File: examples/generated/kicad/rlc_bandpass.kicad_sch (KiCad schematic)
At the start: 5 parts

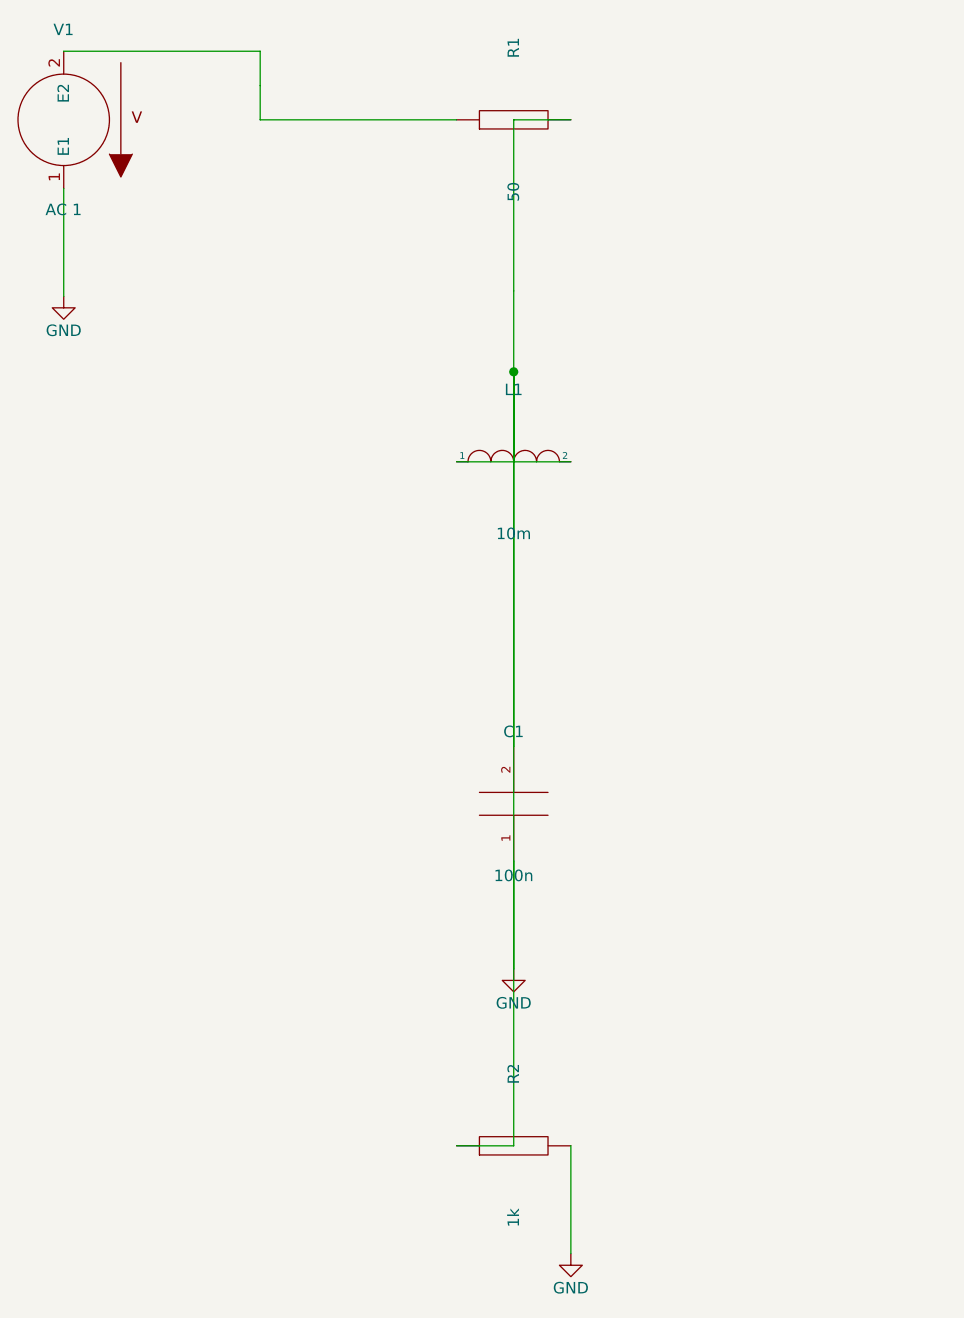
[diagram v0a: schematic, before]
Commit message: Attempt to correct strange wiring.
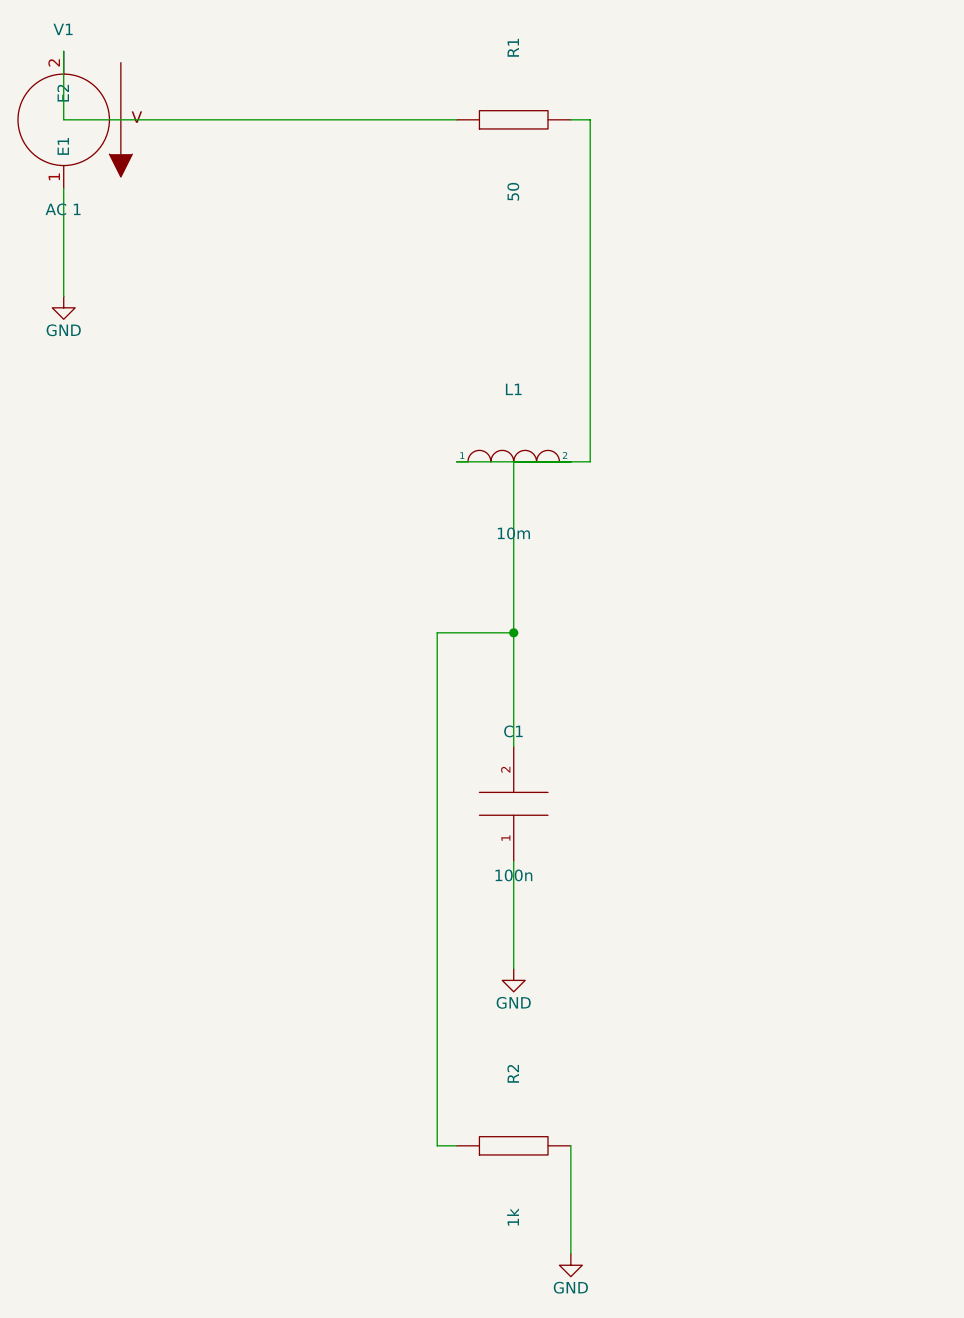
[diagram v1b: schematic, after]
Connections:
- net GND: no longer C1.2, L1.1, L1.2, R1.2, R2.1
- new net: C1.2, L1.1, L1.2, R1.2, R2.1
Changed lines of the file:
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@@
     (stroke (width 0) (type solid) (color 0 0 0 0))
   )
-  (wire (pts (xy 106.35 70.00) (xy 100.00 70.00))
+  (wire (pts (xy 106.35 70.00) (xy 108.50 70.00))
     (stroke (width 0) (type solid) (color 0 0 0 0))
   )
-  (wire (pts (xy 100.00 70.00) (xy 100.00 89.00))
+  (wire (pts (xy 108.50 70.00) (xy 108.50 108.00))
     (stroke (width 0) (type solid) (color 0 0 0 0))
   )
-  (wire (pts (xy 93.65 108.00) (xy 100.00 108.00))
-    (stroke (width 0) (type solid) (color 0 0 0 0))
-  )
-  (wire (pts (xy 100.00 108.00) (xy 100.00 89.00))
+  (wire (pts (xy 108.50 108.00) (xy 93.65 108.00))
     (stroke (width 0) (type solid) (color 0 0 0 0))
   )
@@
     (stroke (width 0) (type solid) (color 0 0 0 0))
   )
-  (wire (pts (xy 100.00 108.00) (xy 100.00 98.00))
+  (wire (pts (xy 100.00 108.00) (xy 100.00 127.00))
     (stroke (width 0) (type solid) (color 0 0 0 0))
   )
-  (wire (pts (xy 100.00 139.65) (xy 100.00 98.00))
+  (wire (pts (xy 100.00 139.65) (xy 100.00 127.00))
     (stroke (width 0) (type solid) (color 0 0 0 0))
   )
-  (wire (pts (xy 93.65 184.00) (xy 100.00 184.00))
+  (wire (pts (xy 93.65 184.00) (xy 91.50 184.00))
     (stroke (width 0) (type solid) (color 0 0 0 0))
   )
-  (wire (pts (xy 100.00 184.00) (xy 100.00 98.00))
+  (wire (pts (xy 91.50 184.00) (xy 91.50 127.00))
     (stroke (width 0) (type solid) (color 0 0 0 0))
   )
-  (wire (pts (xy 50.00 62.38) (xy 71.83 62.38))
+  (wire (pts (xy 91.50 127.00) (xy 100.00 127.00))
     (stroke (width 0) (type solid) (color 0 0 0 0))
   )
-  (wire (pts (xy 71.83 62.38) (xy 71.83 66.19))
+  (wire (pts (xy 50.00 62.38) (xy 50.00 70.00))
     (stroke (width 0) (type solid) (color 0 0 0 0))
   )
-  (wire (pts (xy 93.65 70.00) (xy 71.83 70.00))
+  (wire (pts (xy 50.00 70.00) (xy 93.65 70.00))
     (stroke (width 0) (type solid) (color 0 0 0 0))
   )
-  (wire (pts (xy 71.83 70.00) (xy 71.83 66.19))
-    (stroke (width 0) (type solid) (color 0 0 0 0))
-  )
-  (junction (at 100.00 98.00) (diameter 1.016) (color 0 0 0 0))
+  (junction (at 100.00 127.00) (diameter 1.016) (color 0 0 0 0))
   (sheet_instances
     (path "/" (page "1"))

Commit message: Attempt shape and wiring fixes again.
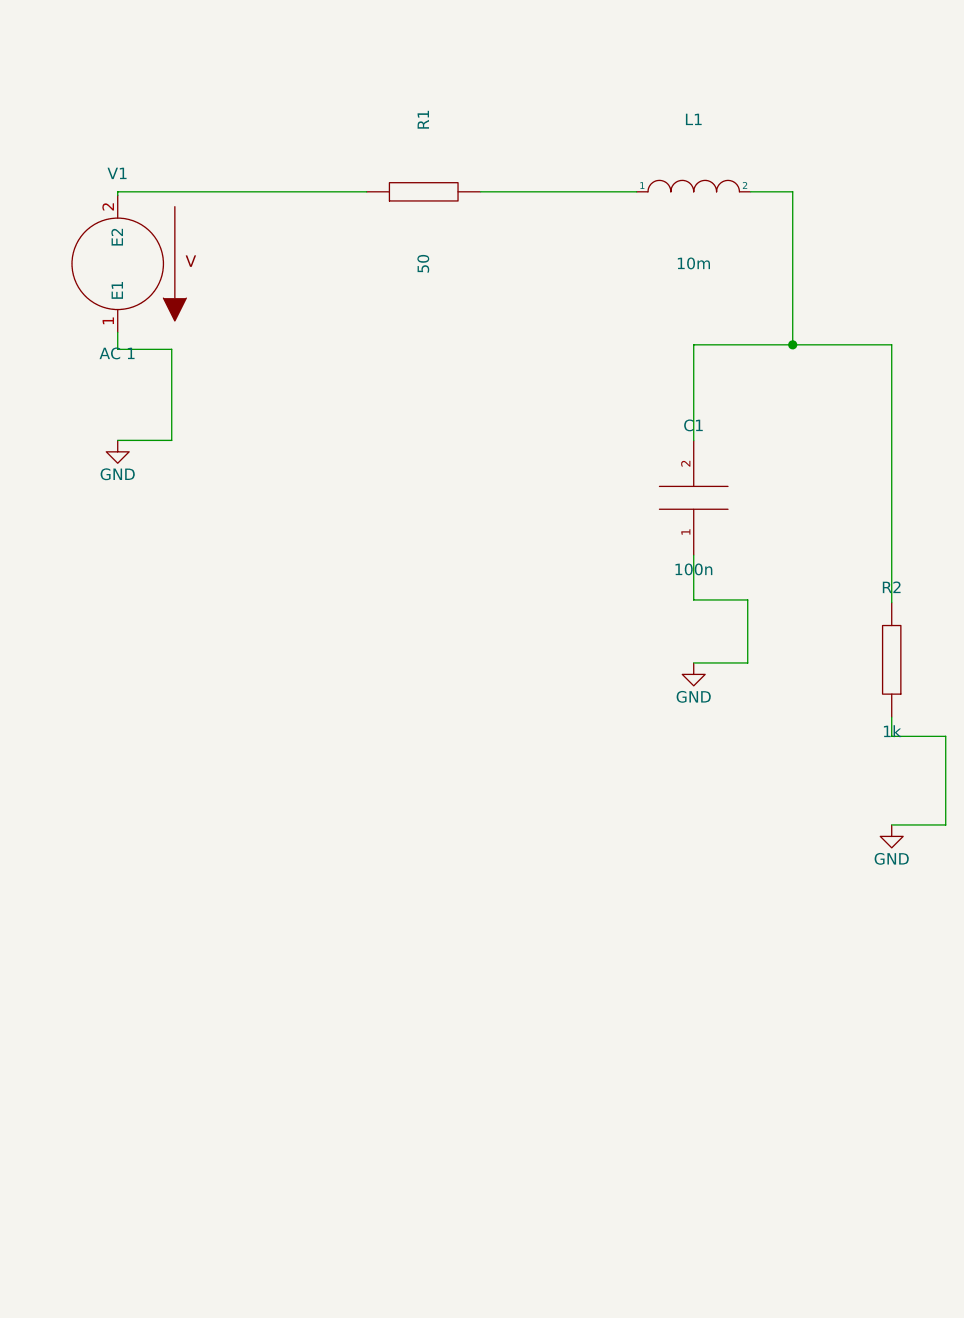
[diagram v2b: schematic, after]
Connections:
- net GND: now also R2.1; no longer R2.2
- new net: L1.1, R1.2
- new net: C1.2, L1.2, R2.2
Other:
- moved on the sheet: C1, L1, R1, R2, V1
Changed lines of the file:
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@@
     (comment 1 "Generated by mixedsig2cad")
   )
-  (symbol (lib_id "VSOURCE") (at 50.00 70.00 180) (unit 1)
+  (symbol (lib_id "VSOURCE") (at 56.00 86.00 180) (unit 1)
     (in_bom yes) (on_board yes)
-    (property "Reference" "V1" (at 50.0 60.0 0)
+    (property "Reference" "V1" (at 56.0 76.0 0)
       (effects (font (size 1.27 1.27)))
     )
-    (property "Value" "AC 1" (at 50.0 80.0 0)
+    (property "Value" "AC 1" (at 56.0 96.0 0)
       (effects (font (size 1.27 1.27)))
     )
@@
     )
   )
-  (symbol (lib_id "R") (at 100.00 70.00 90) (unit 1)
+  (symbol (lib_id "R") (at 90.00 78.00 90) (unit 1)
     (in_bom yes) (on_board yes)
-    (property "Reference" "R1" (at 100.0 62.0 0)
+    (property "Reference" "R1" (at 90.0 70.0 0)
       (effects (font (size 1.27 1.27)))
     )
-    (property "Value" "50" (at 100.0 78.0 0)
+    (property "Value" "50" (at 90.0 86.0 0)
       (effects (font (size 1.27 1.27)))
     )
@@
     )
   )
-  (symbol (lib_id "INDUCTOR") (at 100.00 108.00 0) (unit 1)
+  (symbol (lib_id "INDUCTOR") (at 120.00 78.00 0) (unit 1)
     (in_bom yes) (on_board yes)
-    (property "Reference" "L1" (at 100.0 100.0 0)
+    (property "Reference" "L1" (at 120.0 70.0 0)
       (effects (font (size 1.27 1.27)))
     )
-    (property "Value" "10m" (at 100.0 116.0 0)
+    (property "Value" "10m" (at 120.0 86.0 0)
       (effects (font (size 1.27 1.27)))
     )
@@
     )
   )
-  (symbol (lib_id "CAP") (at 100.00 146.00 180) (unit 1)
+  (symbol (lib_id "CAP") (at 120.00 112.00 180) (unit 1)
     (in_bom yes) (on_board yes)
-    (property "Reference" "C1" (at 100.0 138.0 0)
+    (property "Reference" "C1" (at 120.0 104.0 0)
       (effects (font (size 1.27 1.27)))
     )
-    (property "Value" "100n" (at 100.0 154.0 0)
+    (property "Value" "100n" (at 120.0 120.0 0)
       (effects (font (size 1.27 1.27)))
     )
@@
     )
   )
-  (symbol (lib_id "R") (at 100.00 184.00 90) (unit 1)
+  (symbol (lib_id "R") (at 142.00 130.00 180) (unit 1)
     (in_bom yes) (on_board yes)
-    (property "Reference" "R2" (at 100.0 176.0 0)
+    (property "Reference" "R2" (at 142.0 122.0 0)
       (effects (font (size 1.27 1.27)))
     )
-    (property "Value" "1k" (at 100.0 192.0 0)
+    (property "Value" "1k" (at 142.0 138.0 0)
       (effects (font (size 1.27 1.27)))
     )
@@
     )
   )
-  (symbol (lib_id "GND") (at 50.00 89.62 0) (unit 1)
+  (symbol (lib_id "GND") (at 56.00 105.62 0) (unit 1)
     (in_bom yes) (on_board yes)
-    (property "Reference" "#PWR0001" (at 50.0 85.81 0)
+    (property "Reference" "#PWR0001" (at 56.0 101.81 0)
       (effects (font (size 1.27 1.27)) hide)
     )
-    (property "Value" "GND" (at 50.0 93.43 0)
+    (property "Value" "GND" (at 56.0 109.43 0)
       (effects (font (size 1.27 1.27)))
     )
@@
     )
   )
-  (symbol (lib_id "GND") (at 100.00 164.35 0) (unit 1)
+  (symbol (lib_id "GND") (at 120.00 130.35 0) (unit 1)
     (in_bom yes) (on_board yes)
-    (property "Reference" "#PWR0002" (at 100.0 160.54 0)
+    (property "Reference" "#PWR0002" (at 120.0 126.53999999999999 0)
       (effects (font (size 1.27 1.27)) hide)
     )
-    (property "Value" "GND" (at 100.0 168.16 0)
+    (property "Value" "GND" (at 120.0 134.16 0)
       (effects (font (size 1.27 1.27)))
     )
@@
     )
   )
-  (symbol (lib_id "GND") (at 106.35 196.00 0) (unit 1)
+  (symbol (lib_id "GND") (at 142.00 148.35 0) (unit 1)
     (in_bom yes) (on_board yes)
-    (property "Reference" "#PWR0003" (at 106.35 192.19 0)
+    (property "Reference" "#PWR0003" (at 142.0 144.54 0)
       (effects (font (size 1.27 1.27)) hide)
     )
-    (property "Value" "GND" (at 106.35 199.81 0)
+    (property "Value" "GND" (at 142.0 152.16 0)
       (effects (font (size 1.27 1.27)))
     )
@@
     )
   )
-  (wire (pts (xy 50.00 77.62) (xy 50.00 89.62))
+  (wire (pts (xy 56.00 93.62) (xy 56.00 95.50))
     (stroke (width 0) (type solid) (color 0 0 0 0))
   )
-  (wire (pts (xy 100.00 152.35) (xy 100.00 164.35))
+  (wire (pts (xy 56.00 95.50) (xy 62.00 95.50))
     (stroke (width 0) (type solid) (color 0 0 0 0))
   )
-  (wire (pts (xy 106.35 184.00) (xy 106.35 196.00))
+  (wire (pts (xy 62.00 95.50) (xy 62.00 105.62))
     (stroke (width 0) (type solid) (color 0 0 0 0))
   )
-  (wire (pts (xy 106.35 70.00) (xy 108.50 70.00))
+  (wire (pts (xy 62.00 105.62) (xy 56.00 105.62))
     (stroke (width 0) (type solid) (color 0 0 0 0))
   )
-  (wire (pts (xy 108.50 70.00) (xy 108.50 108.00))
+  (wire (pts (xy 120.00 118.35) (xy 120.00 123.35))
     (stroke (width 0) (type solid) (color 0 0 0 0))
   )
-  (wire (pts (xy 108.50 108.00) (xy 93.65 108.00))
+  (wire (pts (xy 120.00 123.35) (xy 126.00 123.35))
     (stroke (width 0) (type solid) (color 0 0 0 0))
   )
-  (wire (pts (xy 106.35 108.00) (xy 100.00 108.00))
+  (wire (pts (xy 126.00 123.35) (xy 126.00 130.35))
     (stroke (width 0) (type solid) (color 0 0 0 0))
   )
-  (wire (pts (xy 100.00 108.00) (xy 100.00 127.00))
+  (wire (pts (xy 126.00 130.35) (xy 120.00 130.35))
     (stroke (width 0) (type solid) (color 0 0 0 0))
   )
-  (wire (pts (xy 100.00 139.65) (xy 100.00 127.00))
+  (wire (pts (xy 142.00 136.35) (xy 142.00 138.50))
     (stroke (width 0) (type solid) (color 0 0 0 0))
   )
-  (wire (pts (xy 93.65 184.00) (xy 91.50 184.00))
+  (wire (pts (xy 142.00 138.50) (xy 148.00 138.50))
     (stroke (width 0) (type solid) (color 0 0 0 0))
   )
-  (wire (pts (xy 91.50 184.00) (xy 91.50 127.00))
+  (wire (pts (xy 148.00 138.50) (xy 148.00 148.35))
     (stroke (width 0) (type solid) (color 0 0 0 0))
   )
-  (wire (pts (xy 91.50 127.00) (xy 100.00 127.00))
+  (wire (pts (xy 148.00 148.35) (xy 142.00 148.35))
     (stroke (width 0) (type solid) (color 0 0 0 0))
   )
-  (wire (pts (xy 50.00 62.38) (xy 50.00 70.00))
+  (wire (pts (xy 96.35 78.00) (xy 113.65 78.00))
     (stroke (width 0) (type solid) (color 0 0 0 0))
   )
-  (wire (pts (xy 50.00 70.00) (xy 93.65 70.00))
+  (wire (pts (xy 126.35 78.00) (xy 131.00 78.00))
     (stroke (width 0) (type solid) (color 0 0 0 0))
   )
-  (junction (at 100.00 127.00) (diameter 1.016) (color 0 0 0 0))
+  (wire (pts (xy 131.00 78.00) (xy 131.00 95.00))
+    (stroke (width 0) (type solid) (color 0 0 0 0))
+  )
+  (wire (pts (xy 120.00 105.65) (xy 120.00 95.00))
+    (stroke (width 0) (type solid) (color 0 0 0 0))
+  )
+  (wire (pts (xy 120.00 95.00) (xy 131.00 95.00))
+    (stroke (width 0) (type solid) (color 0 0 0 0))
+  )
+  (wire (pts (xy 142.00 123.65) (xy 142.00 95.00))
+    (stroke (width 0) (type solid) (color 0 0 0 0))
+  )
+  (wire (pts (xy 142.00 95.00) (xy 131.00 95.00))
+    (stroke (width 0) (type solid) (color 0 0 0 0))
+  )
+  (wire (pts (xy 56.00 78.38) (xy 56.00 78.00))
+    (stroke (width 0) (type solid) (color 0 0 0 0))
+  )
+  (wire (pts (xy 56.00 78.00) (xy 83.65 78.00))
+    (stroke (width 0) (type solid) (color 0 0 0 0))
+  )
+  (junction (at 131.00 95.00) (diameter 1.016) (color 0 0 0 0))
   (sheet_instances
     (path "/" (page "1"))
